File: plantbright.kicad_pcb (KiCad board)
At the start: 2 copper layers, 33 x 54 mm, 24 parts, among them J1 POWER OUT, J2 USB-C, Q1 AO3400A, Q2 AO3400A, Q3 AO3400A, Q5 AO3400A, SW1 USER 0, U1 XIAO-ESP32-C6

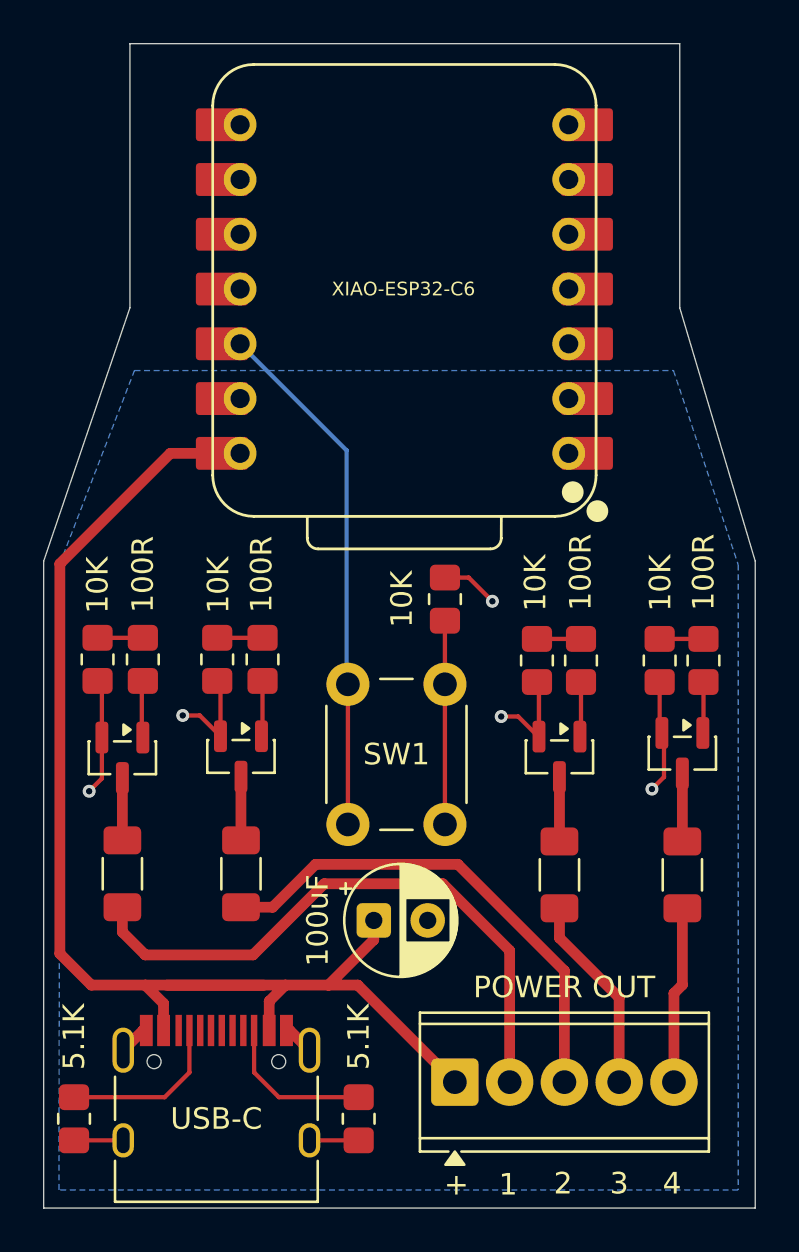
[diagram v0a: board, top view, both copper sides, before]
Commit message: DRC
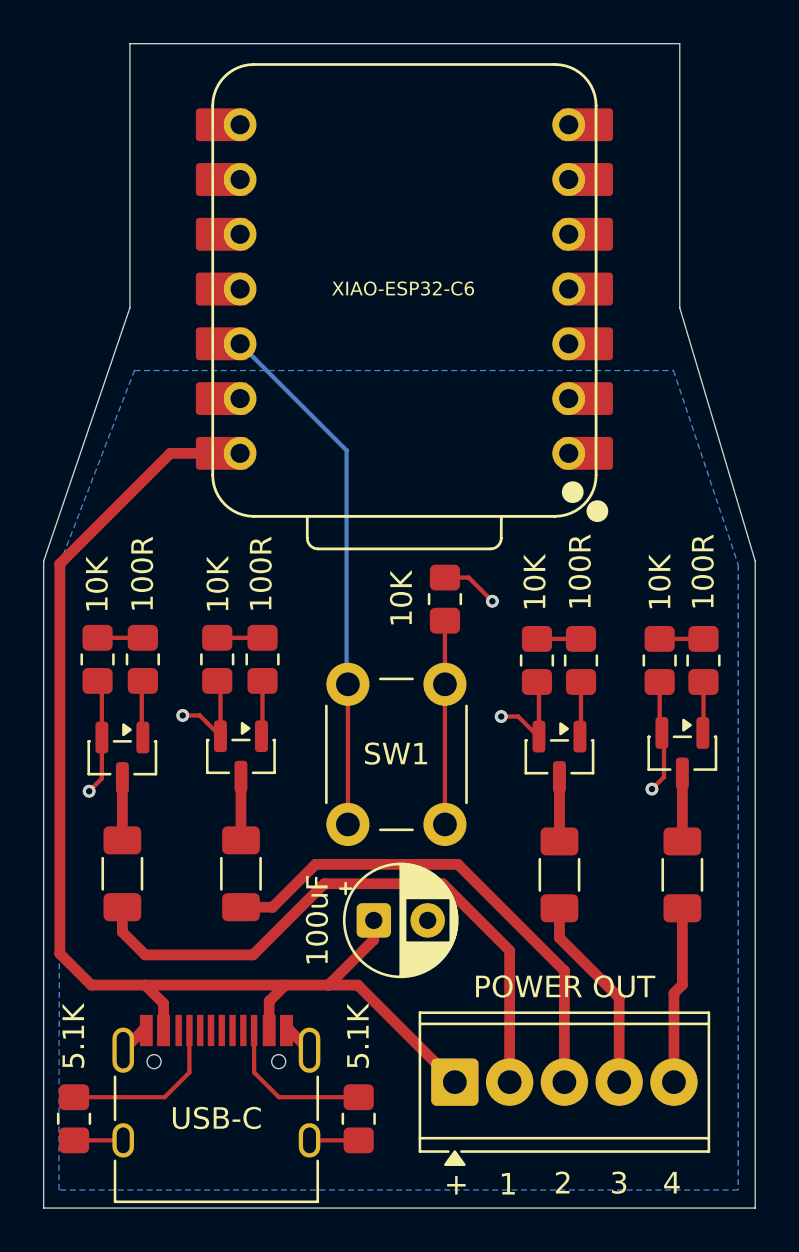
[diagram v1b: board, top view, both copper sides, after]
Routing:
- net +5V: track 62.5 -> 57.3 mm
- net GND: track 30.2 -> 29.5 mm
- net Net-(J1-Pin_5): track 8.78 -> 8.22 mm
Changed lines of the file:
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@@
-	)
-	(segment
-		(start 155.13 112.5)
-		(end 155.86 112.5)
-		(width 0.5)
-		(layer "F.Cu")
-		(net 3)
 	)
 	(segment
@@
 	)
 	(segment
-		(start 147 108)
-		(end 142.5 108)
-		(width 0.5)
-		(layer "F.Cu")
-		(net 3)
-	)
-	(segment
 		(start 152.1 105.9)
 		(end 150 108)
@@
 		(start 144.99 96.45744)
 		(end 144.99 94.04494)
-		(width 0.2)
-		(layer "F.Cu")
-		(net 4)
-	)
-	(segment
-		(start 159.76 94.03744)
-		(end 159.6675 93.94494)
-		(width 0.2)
-		(layer "F.Cu")
-		(net 4)
-	)
-	(segment
-		(start 139.49 94.14494)
-		(end 139.24 93.89494)
-		(width 0.2)
-		(layer "F.Cu")
-		(net 4)
-	)
-	(segment
-		(start 144.99 94.04494)
-		(end 144.84 93.89494)
 		(width 0.2)
 		(layer "F.Cu")
@@
 	)
 	(segment
-		(start 166.41 112.11)
-		(end 166.02 112.5)
-		(width 0.5)
-		(layer "F.Cu")
-		(net 23)
-	)
-	(segment
 		(start 166.02 108.38)
 		(end 166.41 107.99)
@@
 	)
 	(segment
-		(start 145.94 104.38744)
-		(end 145.96256 104.41)
-		(width 0.5)
-		(layer "F.Cu")
-		(net 25)
-	)
-	(segment
